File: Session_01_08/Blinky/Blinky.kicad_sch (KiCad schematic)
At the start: 8 parts

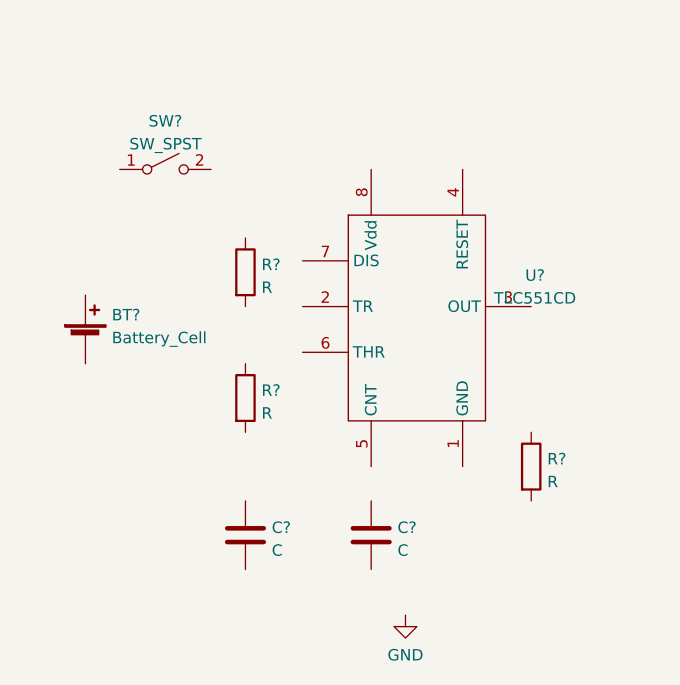
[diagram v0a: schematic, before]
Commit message: Finished the first draft of the work steps
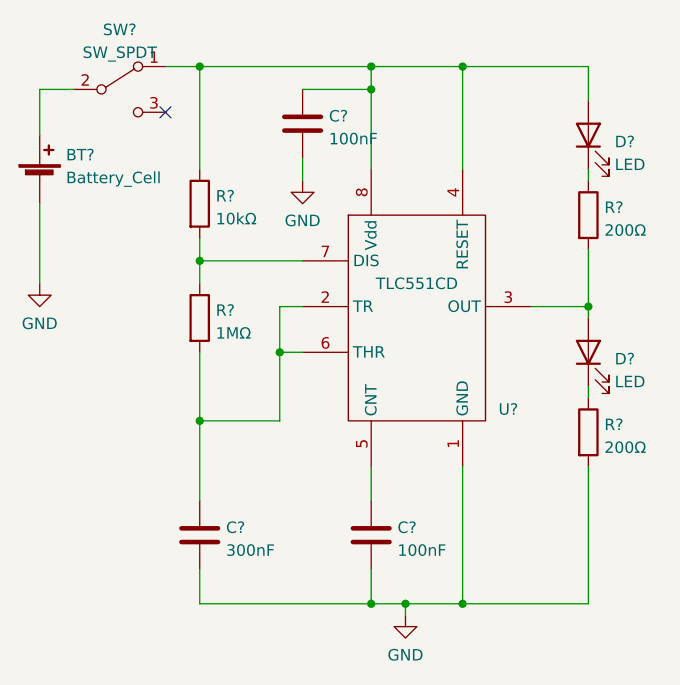
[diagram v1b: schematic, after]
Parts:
- removed SW?: SW_SPST, symbol Switch:SW_SPST
- added C?: 100nF, Capacitor_SMD:C_0805_2012Metric_Pad1.18x1.45mm_HandSolder, symbol Device:C
- added D? (x2): LED, LED_SMD:LED_0805_2012Metric_Pad1.15x1.40mm_HandSolder, symbol Device:LED
- added R?: 200Ω, Resistor_SMD:R_0805_2012Metric_Pad1.20x1.40mm_HandSolder, symbol Device:R
- added SW?: SW_SPDT, Blinky_ZAM:SSK-1202, symbol Switch:SW_SPDT
- BT?: footprint (none) -> Battery:BatteryHolder_Keystone_3000_1x12mm
- C?: value C -> 100nF; footprint (none) -> Capacitor_SMD:C_0805_2012Metric_Pad1.18x1.45mm_HandSolder
- C?: value C -> 300nF; footprint (none) -> Capacitor_SMD:C_0805_2012Metric_Pad1.18x1.45mm_HandSolder
- R?: value R -> 200Ω; footprint (none) -> Resistor_SMD:R_0805_2012Metric_Pad1.20x1.40mm_HandSolder
- R?: value R -> 10kΩ; footprint (none) -> Resistor_SMD:R_0805_2012Metric_Pad1.20x1.40mm_HandSolder
- R?: value R -> 1MΩ; footprint (none) -> Resistor_SMD:R_0805_2012Metric_Pad1.20x1.40mm_HandSolder
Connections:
- net GND: now also BT?.2 (-), C?.2, C?.2, R?.2, U?.1 (GND), C?.2
- net at C?.1: now also U?.5 (CNT)
- net at U?.2 (TR): now also C?.1, R?.2, U?.6 (THR)
- net at U?.3 (OUT): now also D?.2 (A), R?.2
- net at U?.4 (RESET): now also R?.1, U?.8 (Vdd), C?.1, D?.2 (A), SW?.1 (A)
- net at U?.7 (DIS): now also R?.1, R?.2
- net at R?.1: now also D?.1 (K)
- net at BT?.1 (+): now also SW?.2 (B)
- new net: D?.1 (K), R?.1
- no-connect marks 0 -> 1
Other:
- moved on the sheet: BT?, C?, R?
